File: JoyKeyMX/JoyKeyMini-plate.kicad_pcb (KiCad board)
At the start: 2 copper layers, 93 x 51 mm, 13 parts, among them SW1 SW_WITHLED, SW3 SW_WITHLED, SW4 SW_WITHLED, SW5 SW_WITHLED, SW6 SW_WITHLED

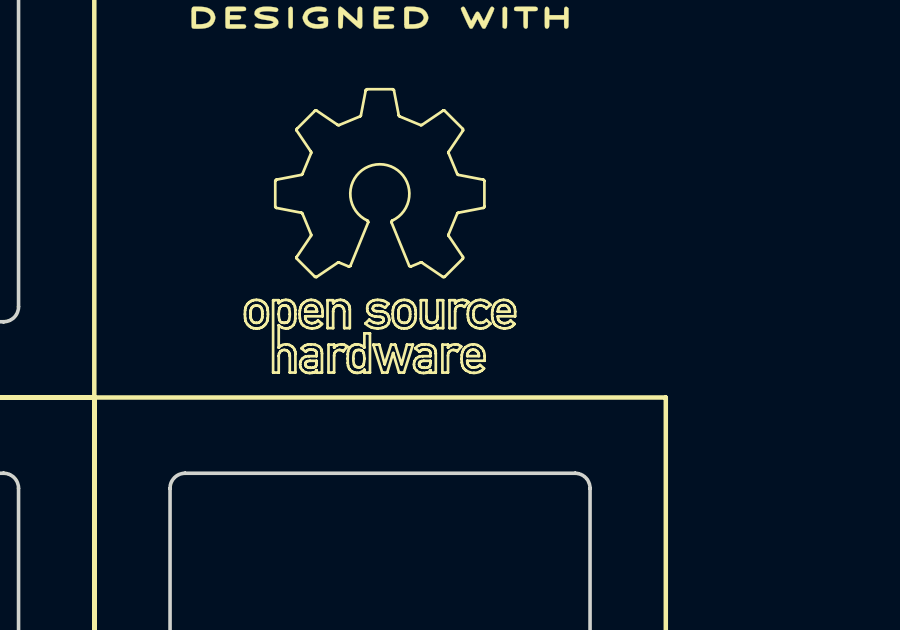
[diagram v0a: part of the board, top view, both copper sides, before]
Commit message: JoyKey Mini PCB and case
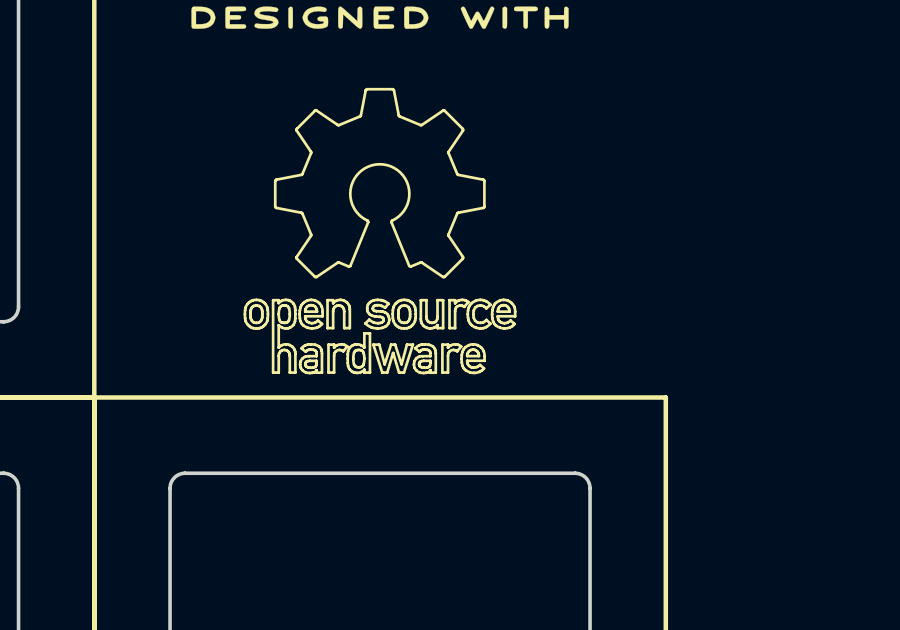
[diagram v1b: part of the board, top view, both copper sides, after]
